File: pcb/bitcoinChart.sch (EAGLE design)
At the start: 29 parts, among them SW5 KMR2, SW6 KMR2, U2 MPU-6050, U7 SPX3819

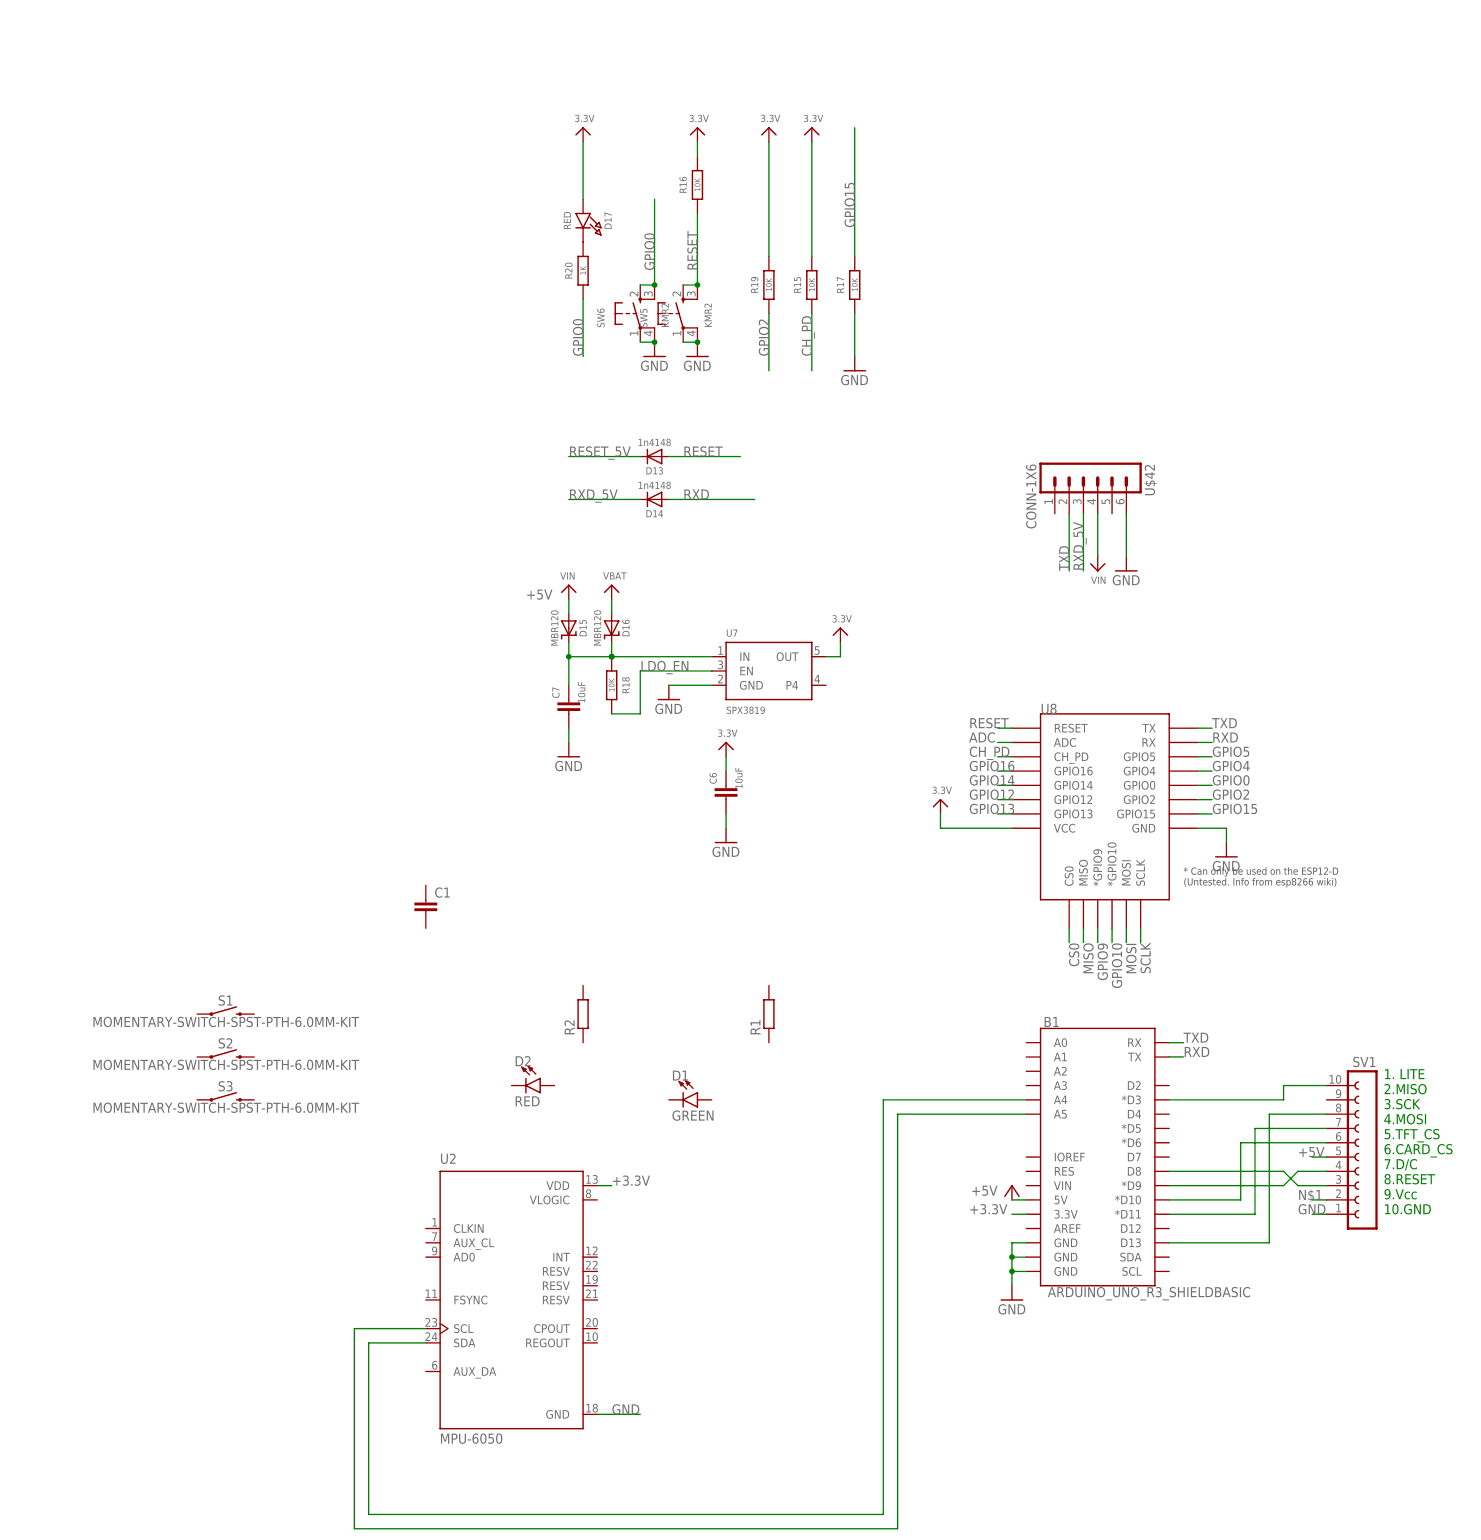
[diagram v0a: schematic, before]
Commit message: Completed PCB
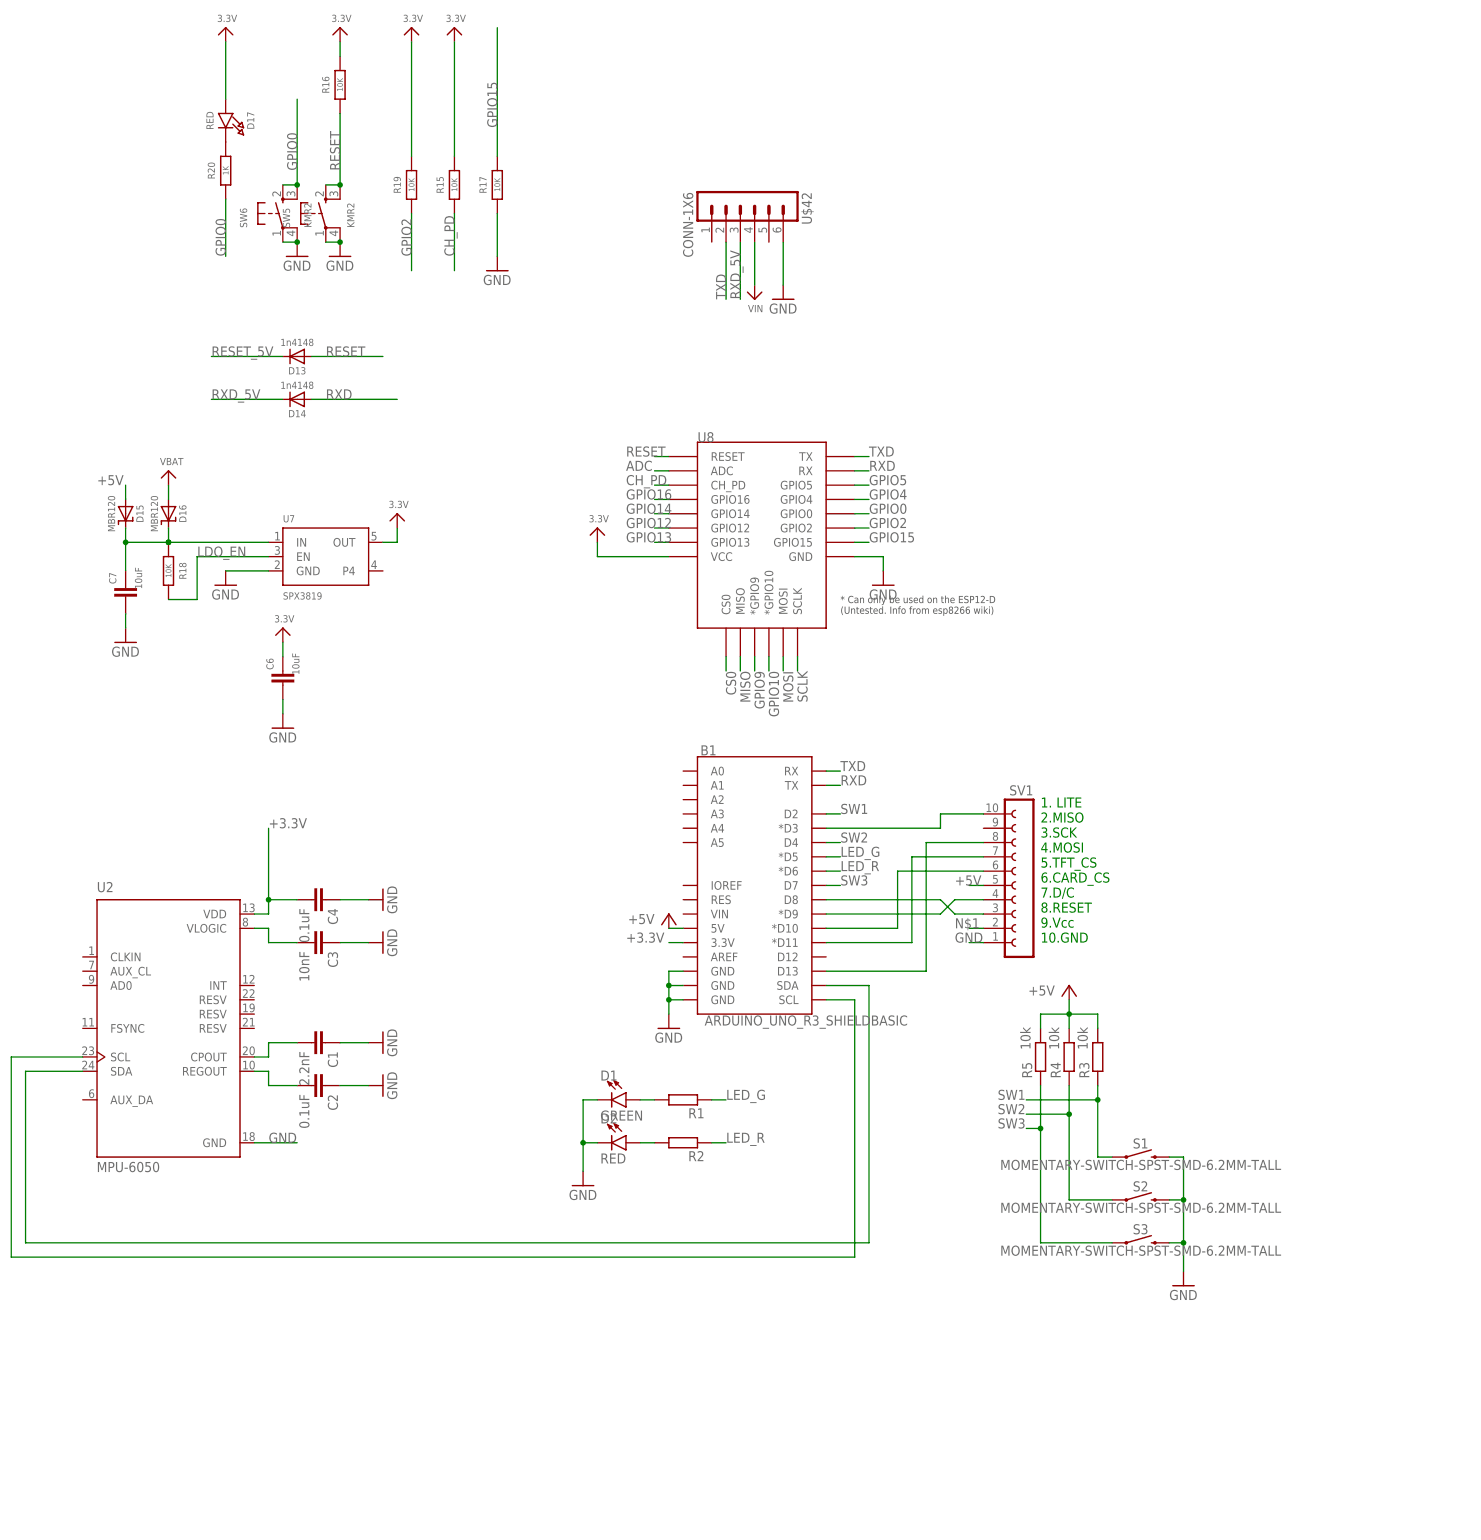
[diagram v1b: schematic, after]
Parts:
- added C2, C4: 0.1uF, resistor:C-EUC1206K
- added C3: 10nF, resistor:C-EUC1206K
- added R3, R4, R5: 10k, resistor:R-EU_M1206
- C1: value (none) -> 2.2nF
- S1, S2, S3: value MOMENTARY-SWITCH-SPST-PTH-6.0MM-KIT -> MOMENTARY-SWITCH-SPST-SMD-6.2MM-TALL; device SparkFun-Switches:MOMENTARY-SWITCH-SPST-PTH-6.0MM-KIT -> SparkFun-Switches:MOMENTARY-SWITCH-SPST-SMD-6.2MM-TALL
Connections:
- new net LED_G: B1.*D5, R1.1
- new net LED_R: B1.*D6, R2.1
- new net N$10: C2.2, U2.REGOUT
- new net N$11: C1.2, U2.CPOUT
- new net N$12: C3.2, U2.VLOGIC
- new net N$13: D1.A, R1.2
- new net N$16: D2.A, R2.2
- new net SW1: B1.D2, R3.1, S1.1
- new net SW2: B1.D4, R4.1, S2.1
- new net SW3: B1.D7, R5.1, S3.1
- net +3.3V: now also C4.2
- net +5V: now also R3.2, R4.2, R5.2
- net GND: now also C1.1, C2.1, C3.1, C4.1, D1.C, D2.C, S1.2, S2.2, S3.2
- net N$2: now also B1.SCL; no longer B1.A5
- net N$3: now also B1.SDA; no longer B1.A4
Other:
- moved on the sheet: B1, C1, C6, C7, D1, D13, D14, D15, D16, D17, D2, R1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
